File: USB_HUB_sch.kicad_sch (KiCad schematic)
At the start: 22 parts, among them IC1 USB2513B_M2, Y1 MURATA_XRCGB24M000FFS1DR0

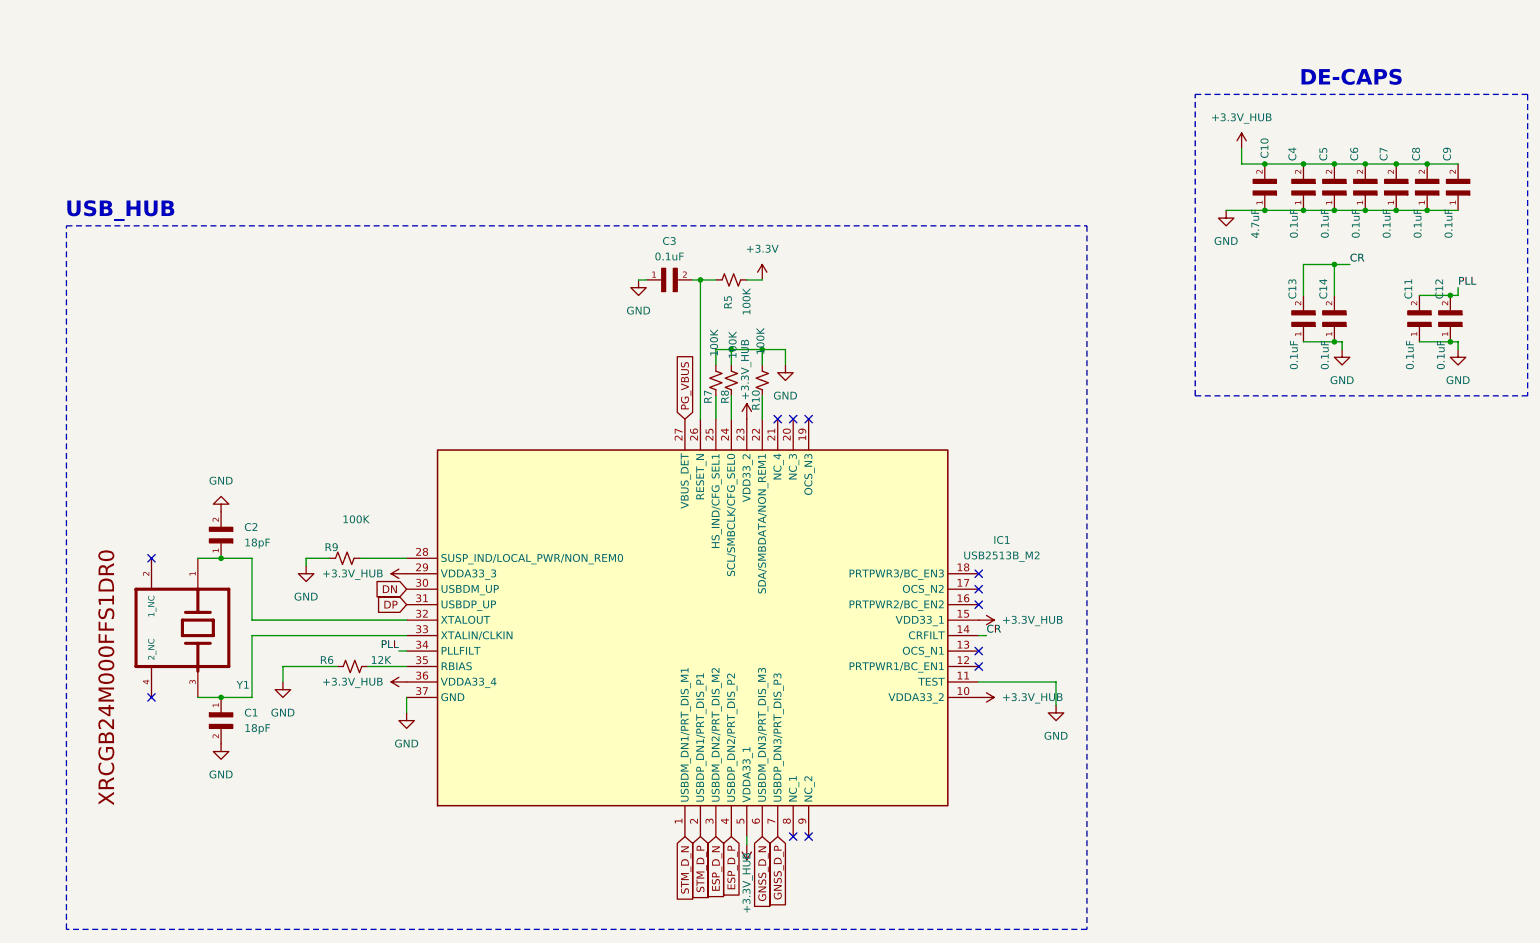
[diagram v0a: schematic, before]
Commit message: new
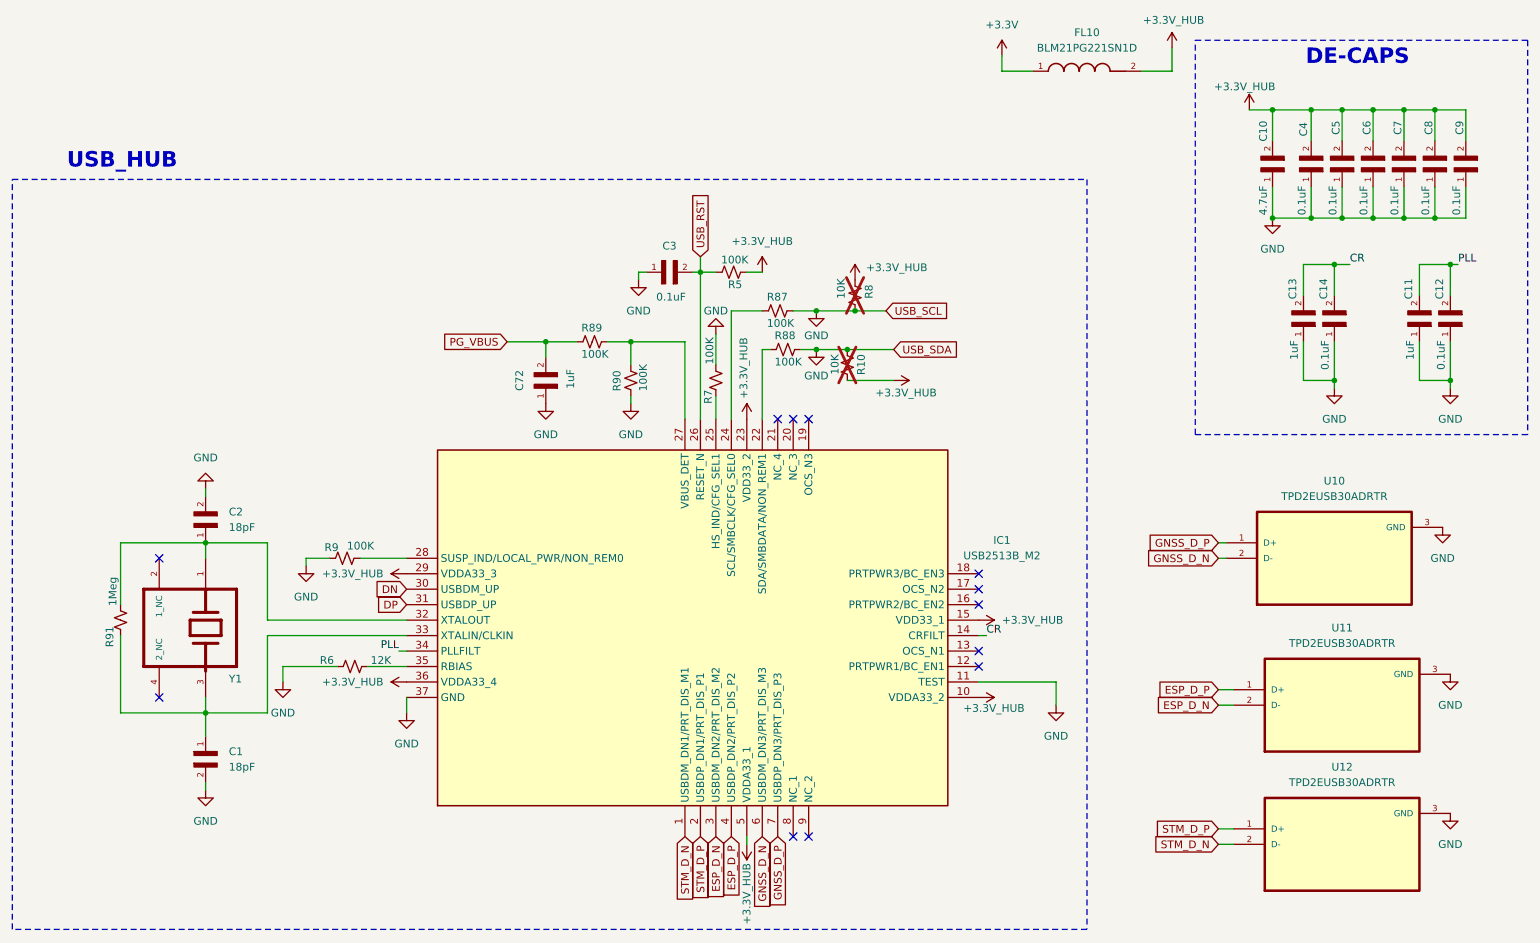
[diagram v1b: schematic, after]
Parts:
- added C72: 1uF, C0402C104K4RAC:CAPC1005X55N, symbol C0402C104K4RAC:C0402C104K4RAC
- added FL10: BLM21PG221SN1D, BLM21PG221SN1D:BEADC2012X105N, symbol BLM21PG221SN1D:BLM21PG221SN1D
- added R87, R88, R89, R90: 100K, Resistor_SMD:R_0402_1005Metric, symbol Device:R_Small_US
- added R91: 1Meg, Resistor_SMD:R_0402_1005Metric, symbol Device:R_Small_US
- added U10, U11, U12: TPD2EUSB30ADRTR, symbol TPD2EUSB30ADRTR:TPD2EUSB30ADRTR
- C11, C13: value 0.1uF -> 1uF
- IC1: footprint QFN50P600X600X100-37N-D -> GNSS:QFN50P600X600X100-37N-D
- R10, R8: value 100K -> 10K; now not fitted
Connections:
- net +3.3V: now also FL10.1; no longer R5.2
- net +3.3V_HUB: now also R10.1, R5.2, R8.2, FL10.2
- net ESP_D_N: now also U11.2 (D-)
- net ESP_D_P: now also U11.1 (D+)
- net GND: now also R8.1, C72.1, R87.1, R88.1, R90.2, U10.3 (GND), U11.3 (GND), U12.3 (GND); no longer R8.2
- net GNSS_D_N: now also U10.2 (D-)
- net GNSS_D_P: now also U10.1 (D+)
- net PG_VBUS: now also C72.2, R89.2; no longer IC1.27 (VBUS_DET)
- net STM_D_N: now also U12.2 (D-)
- net STM_D_P: now also U12.1 (D+)
- net USB_RST: now reaches C3.2, IC1.26 (RESET_N), R5.1
- net at IC1.22 (SDA/SMBDATA/NON_REM1): now also R88.2; no longer R10.1
- net at IC1.24 (SCL/SMBCLK/CFG_SEL0): now also R87.2; no longer R8.1
- net at C2.1, IC1.32 (XTALOUT), Y1.1: now also R91.2
- net at C1.1, IC1.33 (XTALIN/CLKIN), Y1.3: now also R91.1
- new net: IC1.27 (VBUS_DET), R89.1, R90.1
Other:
- moved on the sheet: C1, C10, C2, C3, C4, C5, C6, C7, C8, C9, R5
